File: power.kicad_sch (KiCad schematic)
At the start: 1 part, among them U1 STM32H723ZGTx

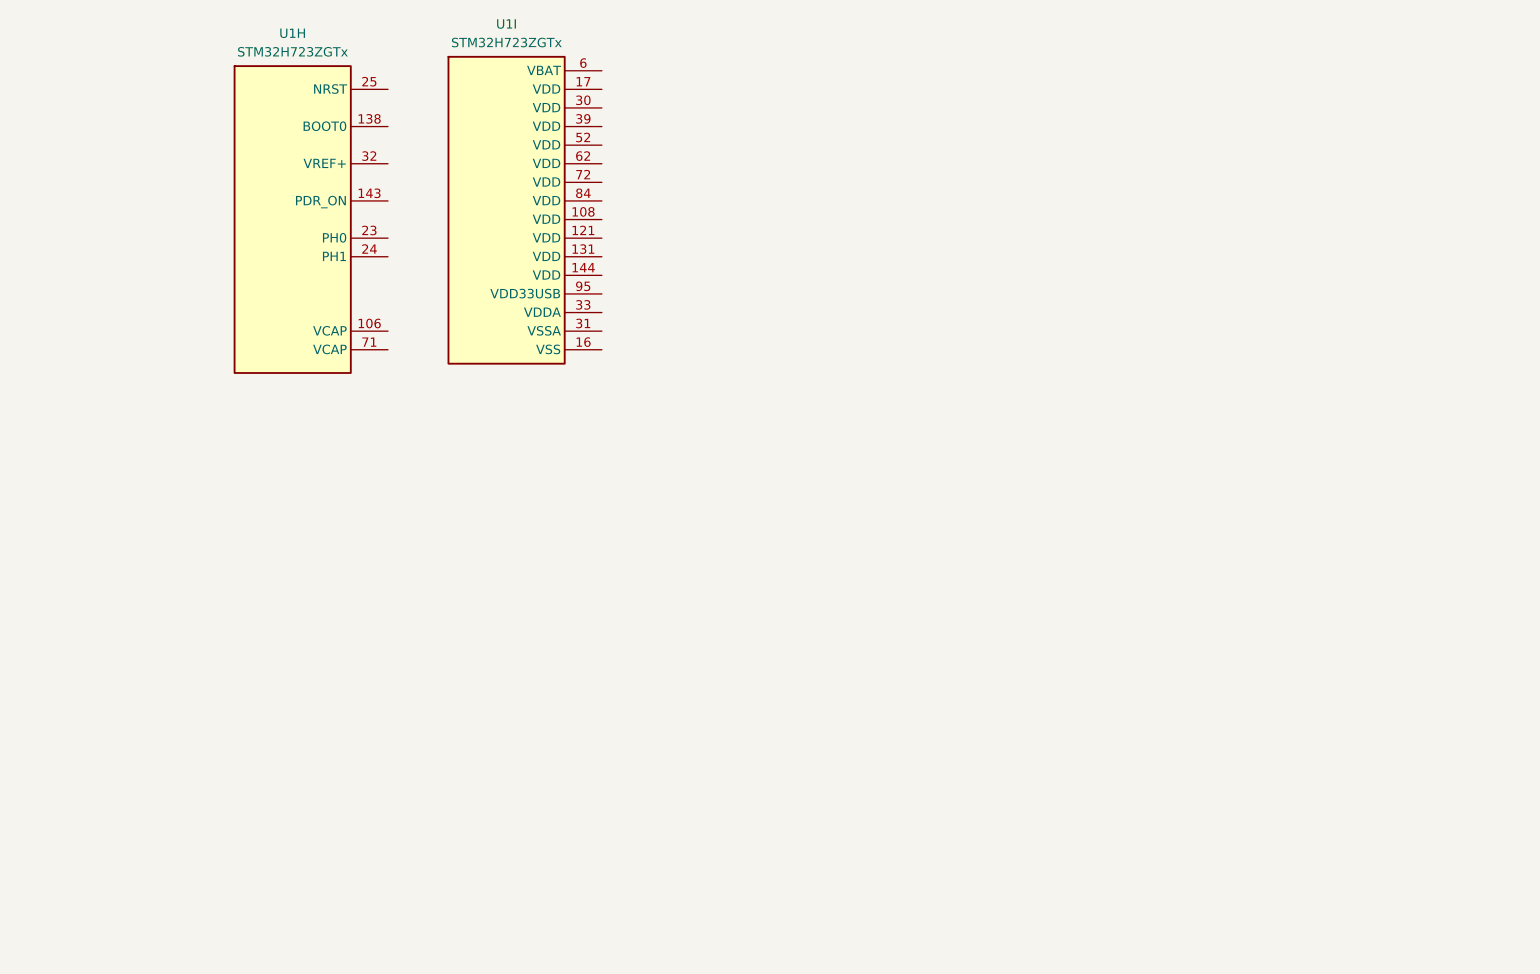
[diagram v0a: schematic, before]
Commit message: I dont know whats going on here
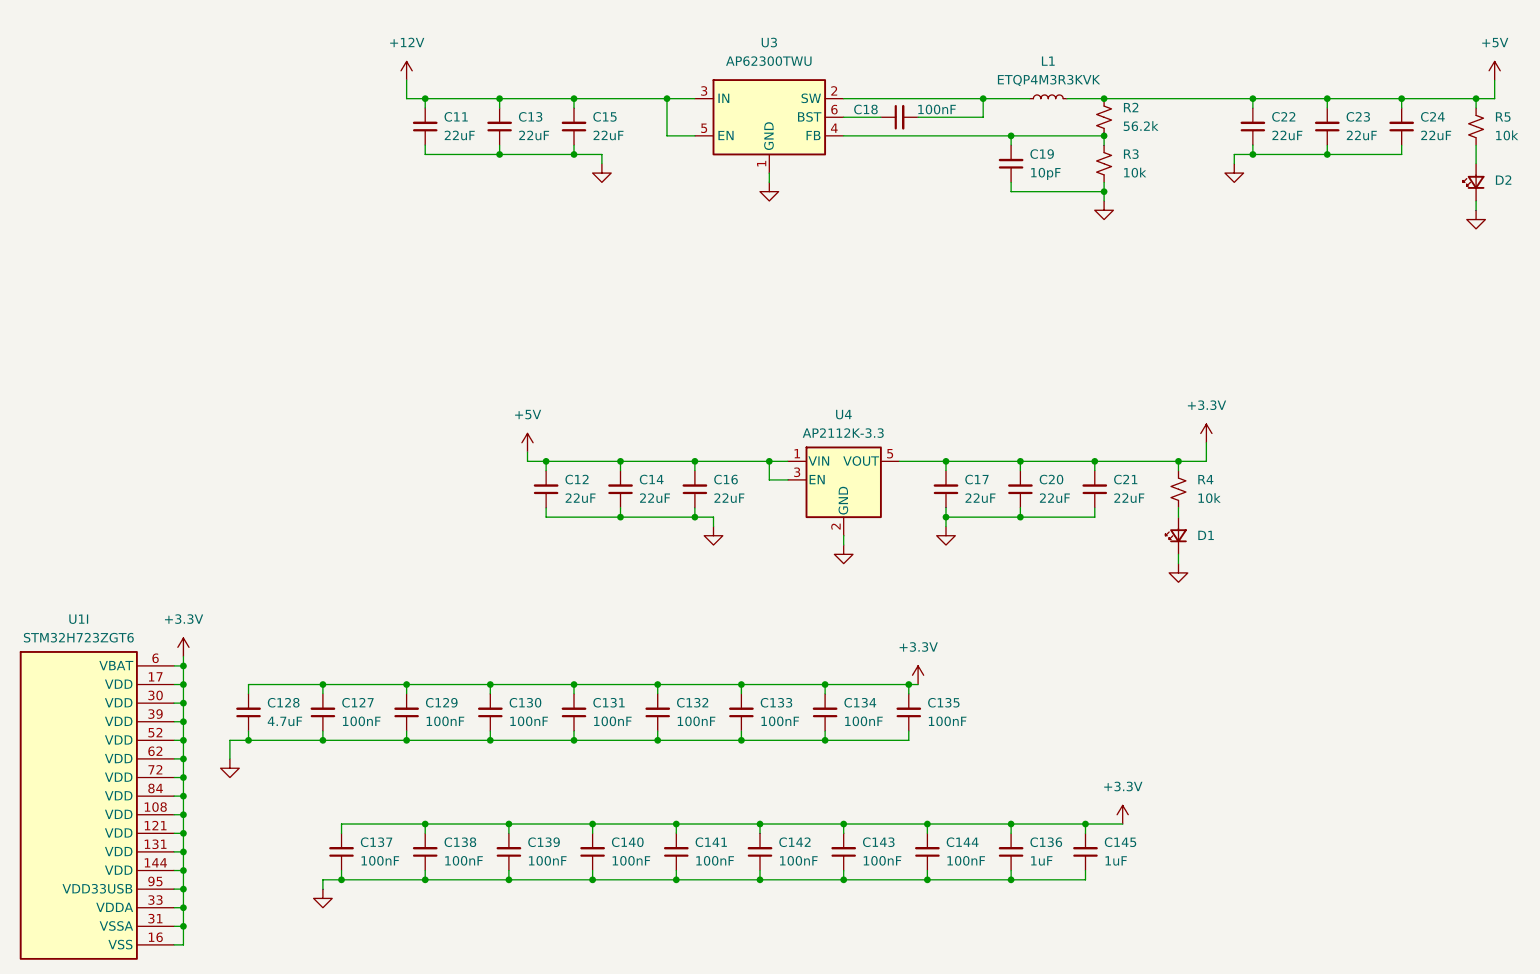
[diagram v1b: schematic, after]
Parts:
- removed unit 8 of U1
- added C11, C12, C13, C14, C15, C16, C17, C20, C21, C22, C23, C24: 22uF, symbol Device:C_Small
- added C127, C129, C130, C131, C132, C133, C134, C135, C137, C138, C139, C140, C141, C142, C143, C144, C18: 100nF, symbol Device:C_Small
- added C128: 4.7uF, symbol Device:C_Small
- added C136, C145: 1uF, symbol Device:C_Small
- added C19: 10pF, symbol Device:C_Small
- added D1, D2: LED_Small, symbol Device:LED_Small
- added L1: ETQP4M3R3KVK, Inductor_SMD:L_Panasonic_PCC-M0850M, symbol Device:L_Small
- added R2: 56.2k, symbol Device:R_Small_US
- added R3, R4, R5: 10k, symbol Device:R_Small_US
- added U3: AP62300TWU, Package_TO_SOT_SMD:TSOT-23-6, symbol Regulator_Switching:AP62300TWU
- added U4: AP2112K-3.3, Package_TO_SOT_SMD:SOT-23-5, symbol Regulator_Linear:AP2112K-3.3
- U1: value STM32H723ZGTx -> STM32H723ZGT6
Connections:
- net +3.3V: now reaches U1.107 (VSS), U1.120 (VSS), U1.130 (VSS), U1.16 (VSS), U1.38 (VSS), U1.51 (VSS), U1.61 (VSS), U1.83 (VSS), U1.94 (VSS)
- net +3.3V: now also U1.108 (VDD), U1.121 (VDD), U1.131 (VDD), U1.144 (VDD), U1.17 (VDD), U1.30 (VDD), U1.31 (VSSA), U1.33 (VDDA), U1.39 (VDD), U1.52 (VDD), U1.6 (VBAT), U1.62 (VDD), U1.72 (VDD), U1.84 (VDD), U1.95 (VDD33USB), C127.2, C128.2, C129.2, C130.2, C131.2, C132.2, C133.2, C134.2, C135.2, C136.2, C137.2, C138.2, C139.2, C140.2, C141.2, C142.2, C143.2, C144.2, C145.2, C17.2, C20.2, C21.2, R4.1, U4.5 (VOUT)
- new net: C19.2, R2.2, R3.1, U3.4 (FB)
- new net: D1.2 (A), R4.2
- new net: C18.1, U3.6 (BST)
- new net: C18.2, L1.1, U3.2 (SW)
- new net: D2.2 (A), R5.2
- new net +12V: C11.2, C13.2, C15.2, U3.3 (IN), U3.5 (EN)
- new net +5V: C12.2, C14.2, C16.2, C22.2, C23.2, C24.2, L1.2, R2.1, R5.1, U4.1 (VIN), U4.3 (EN)
- new net GND: C11.1, C12.1, C127.1, C128.1, C129.1, C13.1, C130.1, C131.1, C132.1, C133.1, C134.1, C135.1, C136.1, C137.1, C138.1, C139.1, C14.1, C140.1, C141.1, C142.1, C143.1, C144.1, C145.1, C15.1, C16.1, C17.1, C19.1, C20.1, C21.1, C22.1, C23.1, C24.1, D1.1 (K), D2.1 (K), R3.2, U3.1 (GND), U4.2 (GND)
